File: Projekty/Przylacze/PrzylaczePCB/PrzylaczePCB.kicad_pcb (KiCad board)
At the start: 2 copper layers, 134.6 x 126 mm, 131 parts, among them J1 Conn_02x20_Odd_Even, J2 USB_B, J3 Conn_01x06, J4 Conn_02x04_Odd_Even, J5 Screw_Terminal_01x06, M3 MountingHole_3.2mm_M3, Q1 BC547, Q10 BC557, Q11 2N3904, Q12 2N7002, Q2 BC547, Q3 BC547, Q4 BC557, Q5 2N3904, Q6 BC557, Q7 BC557, Q8 BC547, Q9 BC557, SW1 SW_Push, SW2 SW_SPDT, SW3 SW_SPDT, SW4 SW_SPDT, SW5 SW_SPDT, SW6 SW_SPDT, SW7 SW_SPDT, SW8 SW_SPDT, SW9 SW_SPDT, U1 MCP2561-E-P, U2 ATSAM4S2AA-AU, U3 MCP2515-xSO, U4 TJA1055T_3_C,518, U5 MAX3485, U6 74AHC1G04, U7 LDL1117S33R, U8 DI78M05UAB, U9 74AHC1G04, Y1 20MHz

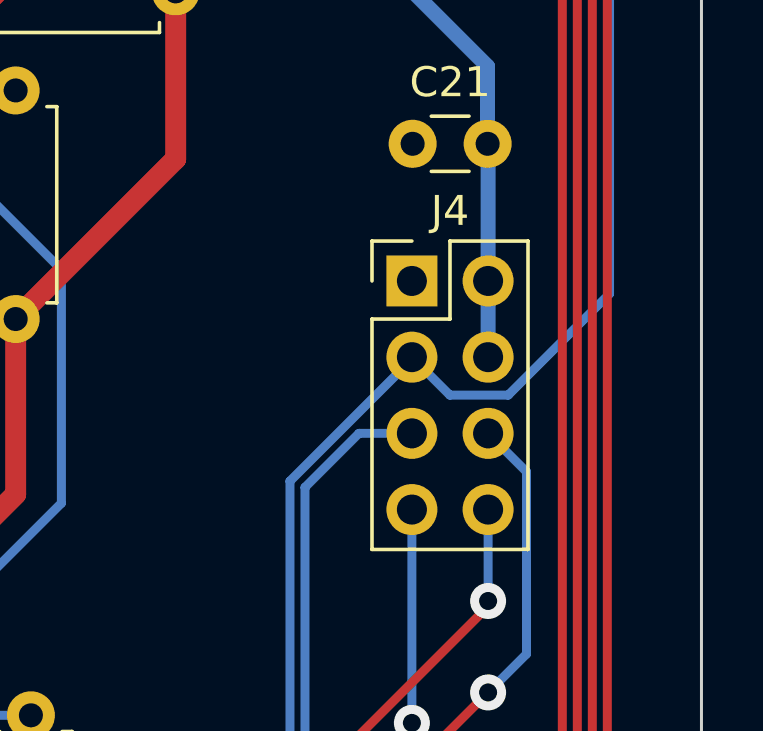
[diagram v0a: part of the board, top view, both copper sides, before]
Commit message: Przyłącze - projekt PCB v1.4.1
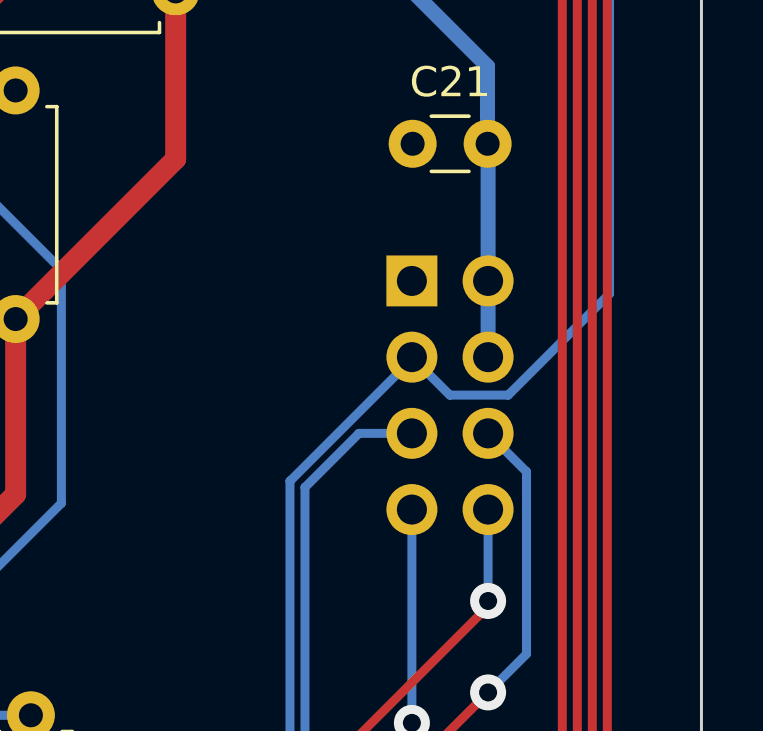
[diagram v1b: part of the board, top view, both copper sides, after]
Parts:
- J4: footprint Connector_PinHeader_2.54mm:PinHeader_2x04_P2.54mm_Vertical -> Connector_PinSocket_2.54mm:PinSocket_2x04_P2.54mm_Vertical; moved to B.Cu
- turned J4 to 180 degrees
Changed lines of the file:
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@@
     )
   )
-  (footprint "Connector_PinHeader_2.54mm:PinHeader_2x04_P2.54mm_Vertical" placed (layer "F.Cu")
-    (at 165.1 161.544)
-    (descr "Through hole straight pin header, 2x04, 2.54mm pitch, double rows")
-    (tags "Through hole pin header THT 2x04 2.54mm double row")
-    (property "Sheetfile" "PrzylaczePCB.kicad_sch")
-    (property "Sheetname" "")
-    (property "ki_description" "Generic connector, double row, 02x04, odd/even pin numbering scheme (row 1 odd numbers, row 2 even numbers), script generated (kicad-library-utils/schlib/autogen/connector/)")
-    (property "ki_keywords" "connector")
-    (attr through_hole)
-    (fp_text reference "J4" (at 1.27 -2.33) (layer "F.SilkS")
-        (effects (font (size 1 1) (thickness 0.15)))
-    )
-    (fp_text value "Conn_02x04_Odd_Even" (at 1.27 9.95) (layer "F.Fab")
-        (effects (font (size 1 1) (thickness 0.15)))
-    )
-    (fp_text user "${REFERENCE}" (at 1.27 3.81 90) (layer "F.Fab")
-        (effects (font (size 1 1) (thickness 0.15)))
-    )
-    (fp_line (start -1.33 -1.33) (end 0 -1.33)
-      (stroke (width 0.12) (type solid)) (layer "F.SilkS"))
-    (fp_line (start -1.33 0) (end -1.33 -1.33)
-      (stroke (width 0.12) (type solid)) (layer "F.SilkS"))
-    (fp_line (start -1.33 1.27) (end -1.33 8.95)
-      (stroke (width 0.12) (type solid)) (layer "F.SilkS"))
-    (fp_line (start -1.33 1.27) (end 1.27 1.27)
-      (stroke (width 0.12) (type solid)) (layer "F.SilkS"))
-    (fp_line (start -1.33 8.95) (end 3.87 8.95)
-      (stroke (width 0.12) (type solid)) (layer "F.SilkS"))
-    (fp_line (start 1.27 -1.33) (end 3.87 -1.33)
-      (stroke (width 0.12) (type solid)) (layer "F.SilkS"))
-    (fp_line (start 1.27 1.27) (end 1.27 -1.33)
-      (stroke (width 0.12) (type solid)) (layer "F.SilkS"))
-    (fp_line (start 3.87 -1.33) (end 3.87 8.95)
-      (stroke (width 0.12) (type solid)) (layer "F.SilkS"))
-    (fp_line (start -1.8 -1.8) (end -1.8 9.4)
-      (stroke (width 0.05) (type solid)) (layer "F.CrtYd"))
-    (fp_line (start -1.8 9.4) (end 4.35 9.4)
-      (stroke (width 0.05) (type solid)) (layer "F.CrtYd"))
-    (fp_line (start 4.35 -1.8) (end -1.8 -1.8)
-      (stroke (width 0.05) (type solid)) (layer "F.CrtYd"))
-    (fp_line (start 4.35 9.4) (end 4.35 -1.8)
-      (stroke (width 0.05) (type solid)) (layer "F.CrtYd"))
-    (fp_line (start -1.27 0) (end 0 -1.27)
-      (stroke (width 0.1) (type solid)) (layer "F.Fab"))
-    (fp_line (start -1.27 8.89) (end -1.27 0)
-      (stroke (width 0.1) (type solid)) (layer "F.Fab"))
-    (fp_line (start 0 -1.27) (end 3.81 -1.27)
-      (stroke (width 0.1) (type solid)) (layer "F.Fab"))
-    (fp_line (start 3.81 -1.27) (end 3.81 8.89)
-      (stroke (width 0.1) (type solid)) (layer "F.Fab"))
-    (fp_line (start 3.81 8.89) (end -1.27 8.89)
-      (stroke (width 0.1) (type solid)) (layer "F.Fab"))
-    (pad "1" thru_hole rect (at 0 0) (size 1.7 1.7) (drill 1) (layers "*.Cu" "*.Mask")
-      (net 1 "GND") (pinfunction "Pin_1") (pintype "passive"))
-    (pad "2" thru_hole oval (at 2.54 0) (size 1.7 1.7) (drill 1) (layers "*.Cu" "*.Mask")
-      (net 2 "+3.3V") (pinfunction "Pin_2") (pintype "passive"))
-    (pad "3" thru_hole oval (at 0 2.54) (size 1.7 1.7) (drill 1) (layers "*.Cu" "*.Mask")
-      (net 31 "CS0") (pinfunction "Pin_3") (pintype "passive"))
-    (pad "4" thru_hole oval (at 2.54 2.54) (size 1.7 1.7) (drill 1) (layers "*.Cu" "*.Mask")
-      (net 2 "+3.3V") (pinfunction "Pin_4") (pintype "passive"))
-    (pad "5" thru_hole oval (at 0 5.08) (size 1.7 1.7) (drill 1) (layers "*.Cu" "*.Mask")
-      (net 32 "SPCK") (pinfunction "Pin_5") (pintype "passive"))
-    (pad "6" thru_hole oval (at 2.54 5.08) (size 1.7 1.7) (drill 1) (layers "*.Cu" "*.Mask")
-      (net 33 "MOSI") (pinfunction "Pin_6") (pintype "passive"))
-    (pad "7" thru_hole oval (at 0 7.62) (size 1.7 1.7) (drill 1) (layers "*.Cu" "*.Mask")
-      (net 34 "MISO") (pinfunction "Pin_7") (pintype "passive"))
-    (pad "8" thru_hole oval (at 2.54 7.62) (size 1.7 1.7) (drill 1) (layers "*.Cu" "*.Mask")
-      (net 35 "RADIO_IRQ") (pinfunction "Pin_8") (pintype "passive"))
-    (model "${KICAD6_3DMODEL_DIR}/Connector_PinHeader_2.54mm.3dshapes/PinHeader_2x04_P2.54mm_Vertical.wrl"
-      (offset (xyz 0 0 0))
-      (scale (xyz 1 1 1))
-      (rotate (xyz 0 0 0))
-    )
-  )
   (footprint "Resistor_THT:R_Axial_DIN0207_L6.3mm_D2.5mm_P10.16mm_Horizontal" placed (layer "F.Cu")
     (at 105.966 103.955 -90)
@@
       (rotate (xyz 0 0 0))
     )
+    (model "${KIPRJMOD}/3DModels/USB-B-S-F-B-TH.stp"
+      (offset (xyz 7 -1.25 0))
+      (scale (xyz 1 1 1))
+      (rotate (xyz 90 180 90))
+    )
   )
   (footprint "Resistor_THT:R_Axial_DIN0207_L6.3mm_D2.5mm_P7.62mm_Horizontal" placed (layer "F.Cu")
@@
     (pad "6" thru_hole circle (at 25.4 0) (size 3 3) (drill 1.5) (layers "*.Cu" "*.Mask")
       (net 1 "GND") (pinfunction "Pin_6") (pintype "passive"))
-    (model "${KICAD6_3DMODEL_DIR}/TerminalBlock.3dshapes/TerminalBlock_bornier-6_P5.08mm.wrl"
+    (model "${KIPRJMOD}/3DModels/TerminalBlock_bornier-6_P5.08mm.wrl"
       (offset (xyz 12.69999981 0 0))
       (scale (xyz 1 1 1))
@@
     )
   )
+  (footprint "Connector_PinSocket_2.54mm:PinSocket_2x04_P2.54mm_Vertical" (layer "B.Cu")
+    (at 165.1 161.544 180)
+    (descr "Through hole straight socket strip, 2x04, 2.54mm pitch, double cols (from Kicad 4.0.7), script generated")
+    (tags "Through hole socket strip THT 2x04 2.54mm double row")
+    (property "Sheetfile" "PrzylaczePCB.kicad_sch")
+    (property "Sheetname" "")
+    (property "ki_description" "Generic connector, double row, 02x04, odd/even pin numbering scheme (row 1 odd numbers, row 2 even numbers), script generated (kicad-library-utils/schlib/autogen/connector/)")
+    (property "ki_keywords" "connector")
+    (attr through_hole)
+    (fp_text reference "J4" (at -1.27 2.77) (layer "B.SilkS")
+        (effects (font (size 1 1) (thickness 0.15)) (justify mirror))
+    )
+    (fp_text value "Conn_02x04_Odd_Even" (at -1.27 -10.39) (layer "B.Fab")
+        (effects (font (size 1 1) (thickness 0.15)) (justify mirror))
+    )
+    (fp_text user "${REFERENCE}" (at -1.27 -3.81 90) (layer "B.Fab")
+        (effects (font (size 1 1) (thickness 0.15)) (justify mirror))
+    )
+    (fp_line (start -3.87 -8.95) (end 1.33 -8.95)
+      (stroke (width 0.12) (type solid)) (layer "B.SilkS"))
+    (fp_line (start -3.87 1.33) (end -3.87 -8.95)
+      (stroke (width 0.12) (type solid)) (layer "B.SilkS"))
+    (fp_line (start -3.87 1.33) (end -1.27 1.33)
+      (stroke (width 0.12) (type solid)) (layer "B.SilkS"))
+    (fp_line (start -1.27 -1.27) (end 1.33 -1.27)
+      (stroke (width 0.12) (type solid)) (layer "B.SilkS"))
+    (fp_line (start -1.27 1.33) (end -1.27 -1.27)
+      (stroke (width 0.12) (type solid)) (layer "B.SilkS"))
+    (fp_line (start 0 1.33) (end 1.33 1.33)
+      (stroke (width 0.12) (type solid)) (layer "B.SilkS"))
+    (fp_line (start 1.33 -1.27) (end 1.33 -8.95)
+      (stroke (width 0.12) (type solid)) (layer "B.SilkS"))
+    (fp_line (start 1.33 1.33) (end 1.33 0)
+      (stroke (width 0.12) (type solid)) (layer "B.SilkS"))
+    (fp_line (start -4.34 -9.4) (end -4.34 1.8)
+      (stroke (width 0.05) (type solid)) (layer "B.CrtYd"))
+    (fp_line (start -4.34 1.8) (end 1.76 1.8)
+      (stroke (width 0.05) (type solid)) (layer "B.CrtYd"))
+    (fp_line (start 1.76 -9.4) (end -4.34 -9.4)
+      (stroke (width 0.05) (type solid)) (layer "B.CrtYd"))
+    (fp_line (start 1.76 1.8) (end 1.76 -9.4)
+      (stroke (width 0.05) (type solid)) (layer "B.CrtYd"))
+    (fp_line (start -3.81 -8.89) (end -3.81 1.27)
+      (stroke (width 0.1) (type solid)) (layer "B.Fab"))
+    (fp_line (start -3.81 1.27) (end 0.27 1.27)
+      (stroke (width 0.1) (type solid)) (layer "B.Fab"))
+    (fp_line (start 0.27 1.27) (end 1.27 0.27)
+      (stroke (width 0.1) (type solid)) (layer "B.Fab"))
+    (fp_line (start 1.27 -8.89) (end -3.81 -8.89)
+      (stroke (width 0.1) (type solid)) (layer "B.Fab"))
+    (fp_line (start 1.27 0.27) (end 1.27 -8.89)
+      (stroke (width 0.1) (type solid)) (layer "B.Fab"))
+    (pad "1" thru_hole rect (at 0 0 180) (size 1.7 1.7) (drill 1) (layers "*.Cu" "*.Mask")
+      (net 1 "GND") (pinfunction "Pin_1") (pintype "passive"))
+    (pad "2" thru_hole oval (at -2.54 0 180) (size 1.7 1.7) (drill 1) (layers "*.Cu" "*.Mask")
+      (net 2 "+3.3V") (pinfunction "Pin_2") (pintype "passive"))
+    (pad "3" thru_hole oval (at 0 -2.54 180) (size 1.7 1.7) (drill 1) (layers "*.Cu" "*.Mask")
+      (net 31 "CS0") (pinfunction "Pin_3") (pintype "passive"))
+    (pad "4" thru_hole oval (at -2.54 -2.54 180) (size 1.7 1.7) (drill 1) (layers "*.Cu" "*.Mask")
+      (net 2 "+3.3V") (pinfunction "Pin_4") (pintype "passive"))
+    (pad "5" thru_hole oval (at 0 -5.08 180) (size 1.7 1.7) (drill 1) (layers "*.Cu" "*.Mask")
+      (net 32 "SPCK") (pinfunction "Pin_5") (pintype "passive"))
+    (pad "6" thru_hole oval (at -2.54 -5.08 180) (size 1.7 1.7) (drill 1) (layers "*.Cu" "*.Mask")
+      (net 33 "MOSI") (pinfunction "Pin_6") (pintype "passive"))
+    (pad "7" thru_hole oval (at 0 -7.62 180) (size 1.7 1.7) (drill 1) (layers "*.Cu" "*.Mask")
+      (net 34 "MISO") (pinfunction "Pin_7") (pintype "passive"))
+    (pad "8" thru_hole oval (at -2.54 -7.62 180) (size 1.7 1.7) (drill 1) (layers "*.Cu" "*.Mask")
+      (net 35 "RADIO_IRQ") (pinfunction "Pin_8") (pintype "passive"))
+    (model "${KICAD6_3DMODEL_DIR}/Connector_PinSocket_2.54mm.3dshapes/PinSocket_2x04_P2.54mm_Vertical.wrl"
+      (offset (xyz 0 0 0))
+      (scale (xyz 1 1 1))
+      (rotate (xyz 0 0 0))
+    )
+  )
   (footprint "PrzylaczeFootprintLibrary:Nexperia-SOT753-10_2018-0-0" placed (layer "B.Cu")
     (at 59.3395 146.3845 -90)
@@
         (xy 118.91 162.15)
         (xy 118.69 161.58)
-        (xy 118.19 161.58)
       )
     )
